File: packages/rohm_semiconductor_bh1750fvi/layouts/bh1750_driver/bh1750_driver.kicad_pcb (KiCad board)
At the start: 2 copper layers, 4 parts

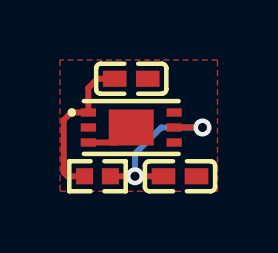
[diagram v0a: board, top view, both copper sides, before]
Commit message: WIP update packages till ESPs
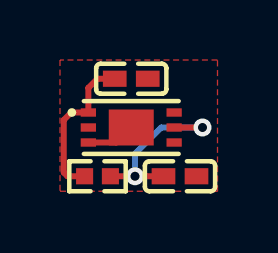
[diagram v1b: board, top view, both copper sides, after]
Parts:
- C1, C2: footprint atopile:C0402-b3ef17 -> Samsung_Electro_Mechanics_CL05B104KO5NNNC:C0402
- R1: footprint atopile:R0402-56259e -> UNI_ROYAL_0402WGF1001TCE:R0402
- U1: footprint atopile:WSOF-6_L2.6-W1.6-P0.50-TL-EP-b2dfd8 -> ROHM_Semicon_BH1750FVI_TR:WSOF-6_L2.6-W1.6-P0.50-TL-EP
